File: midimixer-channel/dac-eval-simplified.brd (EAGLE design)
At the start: 76.2 x 80 mm, 117 parts, among them IC1 NE5534AD, IC2 NE5534AD, IC3 NE5534AD, IC4 NE5534AD, IC5 REG1117-5

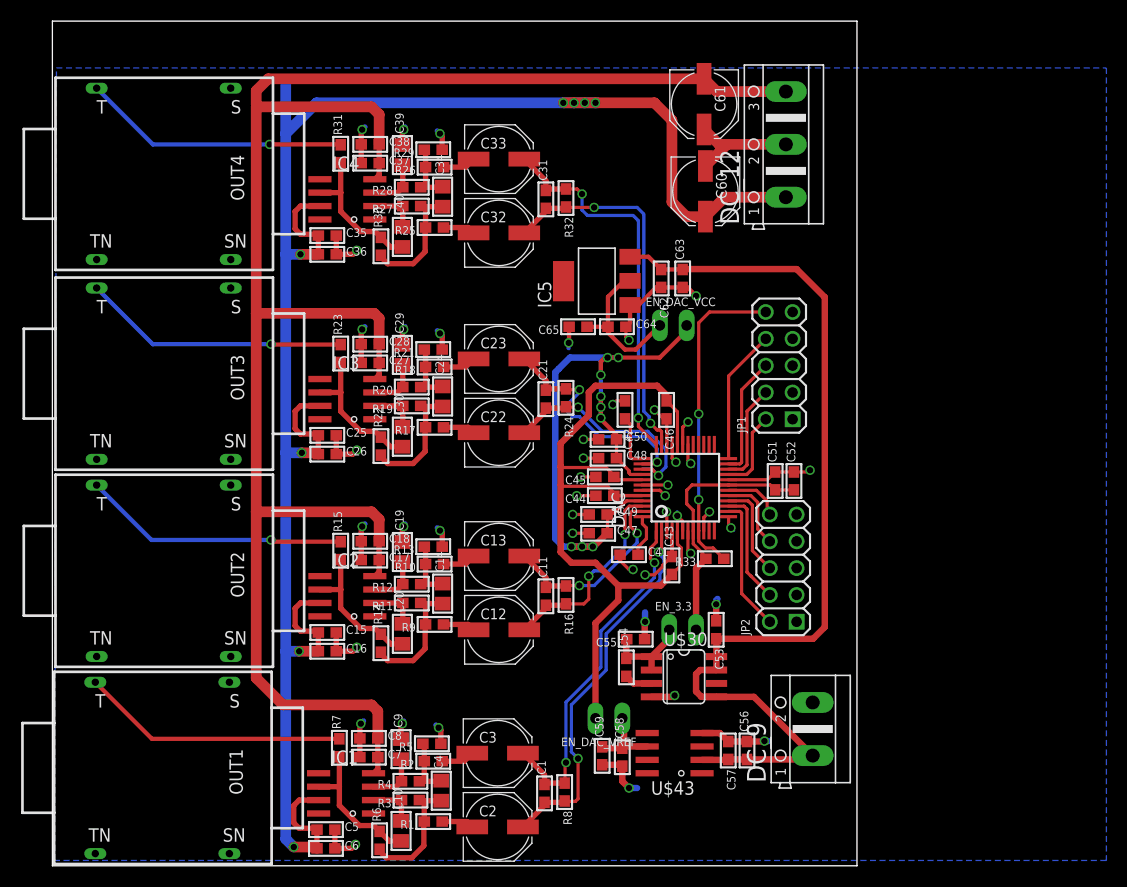
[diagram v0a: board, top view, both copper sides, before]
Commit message: wip
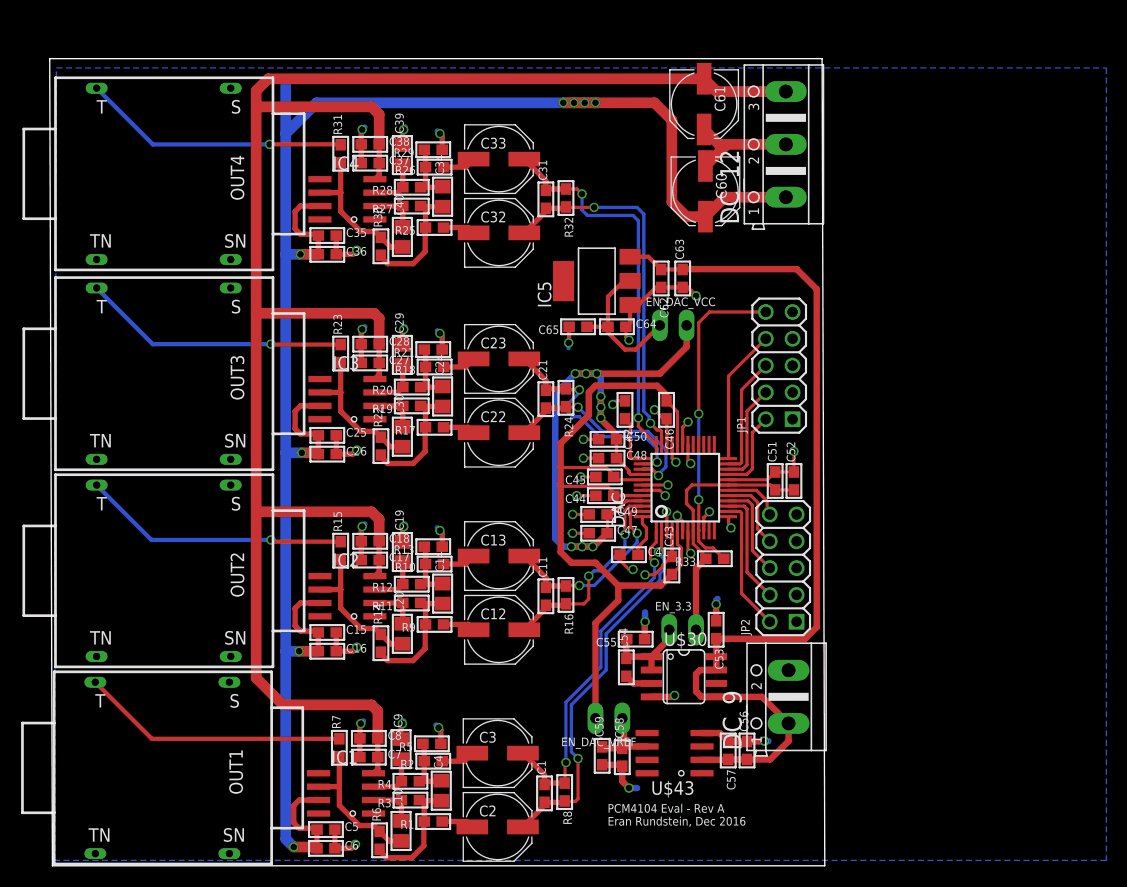
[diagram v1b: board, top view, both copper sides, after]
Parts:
- moved DC_9 3.81 mm to (69.7, 16.0)
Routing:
- net +9V: track 93.0 -> 88.3 mm
- net DAC_VCC: track 62.7 -> 59.8 mm
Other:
- board size 76.2 x 80 mm -> 73.4 x 76.4 mm
- board text added: "PCM4104 Eval - Rev A Eran Rundstein, Dec 2016"
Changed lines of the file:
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@@
 <board>
 <plain>
-<wire x1="0" y1="0" x2="76.2" y2="0" width="0" layer="20"/>
-<wire x1="76.2" y1="0" x2="76.2" y2="80" width="0" layer="20"/>
-<wire x1="76.2" y1="80" x2="0" y2="80" width="0" layer="20"/>
-<wire x1="0" y1="80" x2="0" y2="0" width="0" layer="20"/>
+<wire x1="0" y1="0" x2="73.152" y2="0" width="0" layer="20"/>
+<wire x1="73.152" y1="0" x2="72.898" y2="76.444" width="0" layer="20"/>
+<wire x1="72.898" y1="76.444" x2="-0.254" y2="76.444" width="0" layer="20"/>
+<wire x1="-0.254" y1="76.444" x2="0" y2="0" width="0" layer="20"/>
+<text x="52.578" y="3.81" size="0.8128" layer="21" font="vector">PCM4104 Eval - Rev A
+Eran Rundstein, Dec 2016</text>
 </plain>
 <attributes>
@@
 <attribute name="OC_FARNELL" value="unknown" x="69.469" y="68.326" size="1.778" layer="27" rot="R90" display="off"/>
 </element>
-<element name="DC_9" library="con-ptr500" package="AK500/2" value="" x="72.009" y="12.954" rot="R90">
-<attribute name="MF" value="" x="72.009" y="12.954" size="1.778" layer="27" rot="R90" display="off"/>
-<attribute name="MPN" value="" x="72.009" y="12.954" size="1.778" layer="27" rot="R90" display="off"/>
-<attribute name="OC_NEWARK" value="unknown" x="72.009" y="12.954" size="1.778" layer="27" rot="R90" display="off"/>
-<attribute name="OC_FARNELL" value="unknown" x="72.009" y="12.954" size="1.778" layer="27" rot="R90" display="off"/>
+<element name="DC_9" library="con-ptr500" package="AK500/2" value="" x="69.723" y="16.002" rot="R90">
+<attribute name="MF" value="" x="69.723" y="16.002" size="1.778" layer="27" rot="R90" display="off"/>
+<attribute name="MPN" value="" x="69.723" y="16.002" size="1.778" layer="27" rot="R90" display="off"/>
+<attribute name="OC_NEWARK" value="unknown" x="69.723" y="16.002" size="1.778" layer="27" rot="R90" display="off"/>
+<attribute name="OC_FARNELL" value="unknown" x="69.723" y="16.002" size="1.778" layer="27" rot="R90" display="off"/>
 </element>
 <element name="U$30" library="keves" package="SO08" value="ADP3301ARZ-3.3" x="59.817" y="17.907" rot="R270"/>
@@
 <wire x1="57.873" y1="42.33" x2="57.023" y2="43.18" width="0.3048" layer="1"/>
 <contactref element="DAC" pad="10"/>
-<via x="71.755" y="37.465" extent="1-16" drill="0.6"/>
-<wire x1="70.231" y1="37.299" x2="71.589" y2="37.299" width="0.3048" layer="1"/>
-<wire x1="71.589" y1="37.299" x2="71.755" y2="37.465" width="0.3048" layer="1"/>
+<via x="70.231" y="39.243" extent="1-16" drill="0.6"/>
 <wire x1="60.194" y1="39.914" x2="60.194" y2="38.358" width="0.3048" layer="1"/>
 <wire x1="60.194" y1="38.358" x2="60.452" y2="38.1" width="0.3048" layer="1"/>
@@
 <via x="56.134" y="23.114" extent="1-16" drill="0.6"/>
 <wire x1="56.134" y1="23.114" x2="56.134" y2="24.003" width="0.6096" layer="16"/>
+<wire x1="70.231" y1="37.299" x2="70.231" y2="39.243" width="0.3048" layer="1"/>
 </signal>
 <signal name="3.3V">
@@
 <wire x1="52.666" y1="33.401" x2="52.539" y2="33.274" width="0.3048" layer="1"/>
 <wire x1="53.428" y1="40.386" x2="53.428" y2="40.806" width="0.4064" layer="1"/>
-<wire x1="53.428" y1="40.806" x2="51.943" y2="42.291" width="0.4064" layer="1"/>
+<wire x1="53.428" y1="40.806" x2="51.943" y2="42.291" width="0.6096" layer="1"/>
 <wire x1="51.943" y1="42.291" x2="51.943" y2="42.418" width="0.4064" layer="1"/>
 <via x="51.943" y="44.45" extent="1-16" drill="0.6"/>
-<wire x1="51.943" y1="42.418" x2="51.943" y2="43.434" width="0.4064" layer="1"/>
-<wire x1="51.943" y1="43.434" x2="51.943" y2="44.45" width="0.4064" layer="1"/>
-<wire x1="51.943" y1="44.45" x2="51.943" y2="43.434" width="0.4064" layer="16"/>
-<wire x1="51.943" y1="43.434" x2="51.943" y2="42.418" width="0.4064" layer="16"/>
-<wire x1="51.943" y1="44.45" x2="51.943" y2="46.482" width="0.4064" layer="16"/>
-<wire x1="51.943" y1="46.482" x2="51.943" y2="47.752" width="0.4064" layer="16"/>
-<wire x1="51.943" y1="47.752" x2="52.324" y2="48.133" width="0.4064" layer="16"/>
-<wire x1="52.324" y1="48.133" x2="52.578" y2="48.133" width="0.4064" layer="16"/>
-<wire x1="52.578" y1="48.133" x2="53.594" y2="48.133" width="0.4064" layer="16"/>
-<via x="53.594" y="48.133" extent="1-16" drill="0.6"/>
-<via x="52.578" y="48.133" extent="1-16" drill="0.6"/>
+<wire x1="51.943" y1="42.418" x2="51.943" y2="43.434" width="0.6096" layer="1"/>
+<wire x1="51.943" y1="43.434" x2="51.943" y2="44.45" width="0.6096" layer="1"/>
+<wire x1="51.943" y1="44.45" x2="51.943" y2="43.434" width="0.6096" layer="16"/>
+<wire x1="51.943" y1="43.434" x2="51.943" y2="42.418" width="0.6096" layer="16"/>
+<wire x1="51.943" y1="44.45" x2="51.943" y2="46.609" width="0.6096" layer="16"/>
 <via x="51.943" y="43.434" extent="1-16" drill="0.6"/>
 <via x="51.943" y="42.418" extent="1-16" drill="0.6"/>
-<wire x1="60.071" y1="50.673" x2="60.071" y2="51.181" width="0.4064" layer="1"/>
-<wire x1="53.594" y1="48.133" x2="52.324" y2="48.133" width="0.4064" layer="1"/>
-<wire x1="52.324" y1="48.133" x2="51.943" y2="47.752" width="0.4064" layer="1"/>
-<wire x1="51.943" y1="47.752" x2="51.943" y2="46.482" width="0.4064" layer="1"/>
-<via x="51.943" y="46.482" extent="1-16" drill="0.6"/>
-<wire x1="53.594" y1="48.133" x2="57.531" y2="48.133" width="0.4064" layer="1"/>
-<wire x1="57.531" y1="48.133" x2="60.071" y2="50.673" width="0.4064" layer="1"/>
+<wire x1="49.53" y1="46.609" x2="50.546" y2="46.609" width="0.6096" layer="1"/>
+<wire x1="50.546" y1="46.609" x2="51.562" y2="46.609" width="0.6096" layer="1"/>
+<wire x1="51.562" y1="46.609" x2="57.531" y2="46.609" width="0.6096" layer="1"/>
 <wire x1="52.539" y1="31.496" x2="51.269" y2="30.226" width="0.6096" layer="1"/>
 <wire x1="51.269" y1="30.226" x2="51.181" y2="30.226" width="0.6096" layer="1"/>
@@
 <wire x1="50.165" y1="30.226" x2="49.149" y2="30.226" width="0.6096" layer="1"/>
 <wire x1="48.387" y1="30.226" x2="47.625" y2="30.988" width="0.6096" layer="16"/>
-<wire x1="47.9425" y1="47.0535" x2="49.022" y2="48.133" width="0.6096" layer="16"/>
-<wire x1="49.022" y1="48.133" x2="52.578" y2="48.133" width="0.6096" layer="16"/>
+<wire x1="49.53" y1="46.609" x2="50.546" y2="46.609" width="0.6096" layer="16"/>
+<wire x1="50.546" y1="46.609" x2="51.562" y2="46.609" width="0.6096" layer="16"/>
+<wire x1="51.562" y1="46.609" x2="51.943" y2="46.609" width="0.6096" layer="16"/>
 <wire x1="48.387" y1="30.226" x2="50.165" y2="30.226" width="0.6096" layer="16"/>
 <wire x1="50.165" y1="30.226" x2="51.181" y2="30.226" width="0.6096" layer="16"/>
@@
 <via x="51.181" y="30.226" extent="1-16" drill="0.6"/>
 <via x="50.165" y="30.226" extent="1-16" drill="0.6"/>
-<wire x1="47.625" y1="30.988" x2="47.625" y2="46.736" width="0.6096" layer="16"/>
-<wire x1="47.625" y1="46.736" x2="47.9425" y2="47.0535" width="0.6096" layer="16"/>
+<wire x1="47.625" y1="30.988" x2="47.625" y2="43.815" width="0.6096" layer="16"/>
+<via x="49.53" y="46.609" extent="1-16" drill="0.6"/>
+<via x="50.546" y="46.609" extent="1-16" drill="0.6"/>
+<via x="51.562" y="46.609" extent="1-16" drill="0.6"/>
+<wire x1="47.625" y1="43.815" x2="47.625" y2="44.196" width="0.6096" layer="16"/>
+<wire x1="49.53" y1="46.609" x2="47.625" y2="44.704" width="0.6096" layer="16"/>
+<wire x1="47.625" y1="44.704" x2="47.625" y2="44.196" width="0.6096" layer="16"/>
+<wire x1="57.531" y1="46.609" x2="60.071" y2="49.149" width="0.6096" layer="1"/>
+<wire x1="60.071" y1="49.149" x2="60.071" y2="51.181" width="0.6096" layer="1"/>
 </signal>
 <signal name="+9V">
@@
 <wire x1="63.969" y1="10.033" x2="64.008" y2="10.072" width="0.6096" layer="1"/>
 <wire x1="64.008" y1="10.072" x2="65.786" y2="10.072" width="0.6096" layer="1"/>
-<wire x1="65.786" y1="10.072" x2="71.6416" y2="10.072" width="0.6096" layer="1"/>
-<wire x1="71.6416" y1="10.072" x2="72.009" y2="10.4394" width="0.6096" layer="1"/>
-<wire x1="62.8904" y1="16.002" x2="66.4464" y2="16.002" width="0.6096" layer="1"/>
-<wire x1="66.4464" y1="16.002" x2="72.009" y2="10.4394" width="0.6096" layer="1"/>
-<wire x1="62.865" y1="21.502" x2="72.048" y2="21.502" width="0.6096" layer="1"/>
-<wire x1="72.048" y1="21.502" x2="73.152" y2="22.606" width="0.6096" layer="1"/>
-<wire x1="73.152" y1="22.606" x2="73.152" y2="53.848" width="0.6096" layer="1"/>
-<wire x1="73.152" y1="53.848" x2="70.485" y2="56.515" width="0.6096" layer="1"/>
+<wire x1="62.8904" y1="16.002" x2="67.2084" y2="16.002" width="0.6096" layer="1"/>
+<wire x1="62.865" y1="21.502" x2="71.286" y2="21.502" width="0.6096" layer="1"/>
+<wire x1="72.39" y1="54.61" x2="70.485" y2="56.515" width="0.6096" layer="1"/>
 <wire x1="70.485" y1="56.515" x2="59.729" y2="56.515" width="0.6096" layer="1"/>
 <wire x1="59.729" y1="56.515" x2="59.69" y2="56.476" width="0.6096" layer="1"/>
+<wire x1="71.286" y1="21.502" x2="72.39" y2="22.606" width="0.6096" layer="1"/>
+<wire x1="72.39" y1="22.606" x2="72.39" y2="54.61" width="0.6096" layer="1"/>
+<wire x1="65.786" y1="10.072" x2="67.984" y2="10.072" width="0.6096" layer="1"/>
+<wire x1="67.984" y1="10.072" x2="69.723" y2="11.811" width="0.6096" layer="1"/>
+<wire x1="69.723" y1="11.811" x2="69.723" y2="13.4874" width="0.6096" layer="1"/>
+<wire x1="69.723" y1="13.4874" x2="67.2084" y2="16.002" width="0.6096" layer="1"/>
 </signal>
 <signal name="N$47">
@@
 </board>
 </drawing>
+<compatibility>
+<note version="6.3" minversion="6.2.2" severity="warning">
+Since Version 6.2.2 text objects can contain more than one line,
+which will not be processed correctly with this version.
+</note>
+</compatibility>
 </eagle>
